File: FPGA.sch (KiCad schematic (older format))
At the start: 10 parts, among them U13 ADS1015, U14 SiT8008B, U8 GW1N-9LQ100

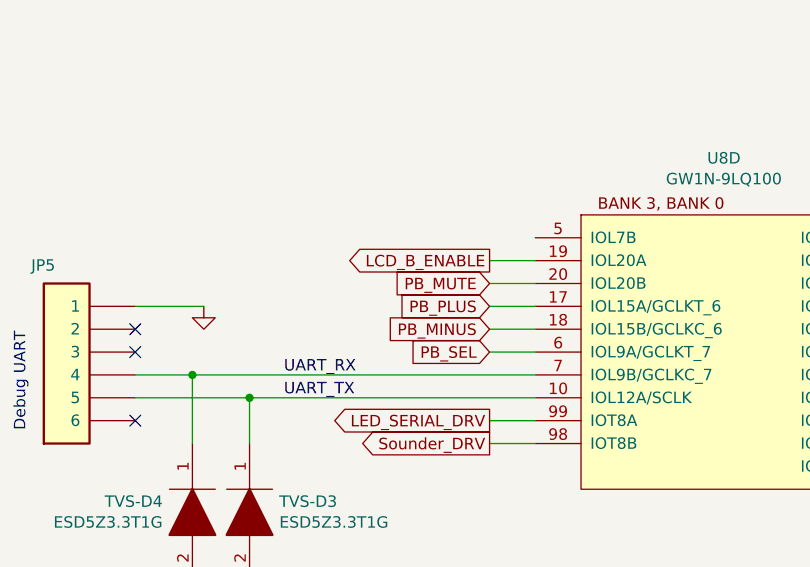
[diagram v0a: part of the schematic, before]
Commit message: Update FPGA.sch
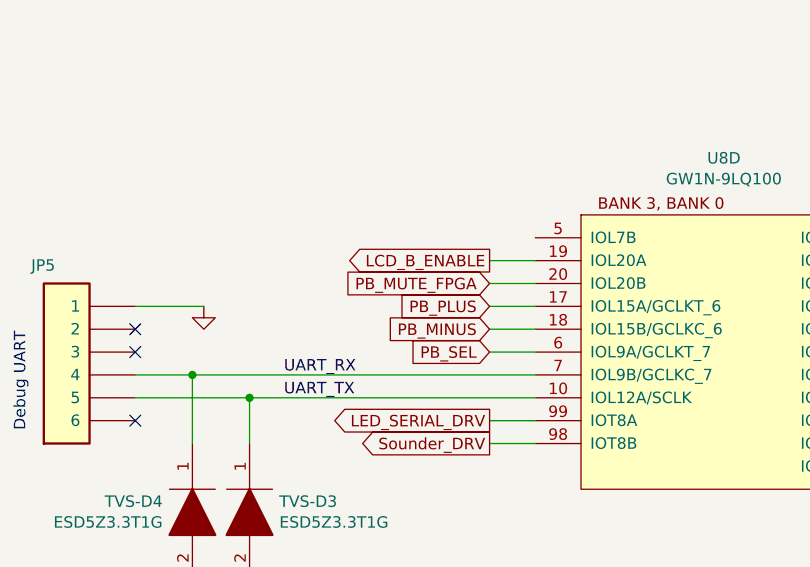
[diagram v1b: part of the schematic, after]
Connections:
- net labels added: PB_MUTE_FPGA
- net labels removed: PB_MUTE
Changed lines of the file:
@@
 Text GLabel 5550 7350 0    50   Output ~ 0
 Motor_off
-Text GLabel 7450 5050 0    50   Input ~ 0
-PB_MUTE
 Text GLabel 7450 5150 0    50   Input ~ 0
 PB_PLUS
@@
 Wire Wire Line
 	6300 6350 6400 6350
+Text GLabel 7450 5050 0    50   Input ~ 0
+PB_MUTE_FPGA
 $EndSCHEMATC

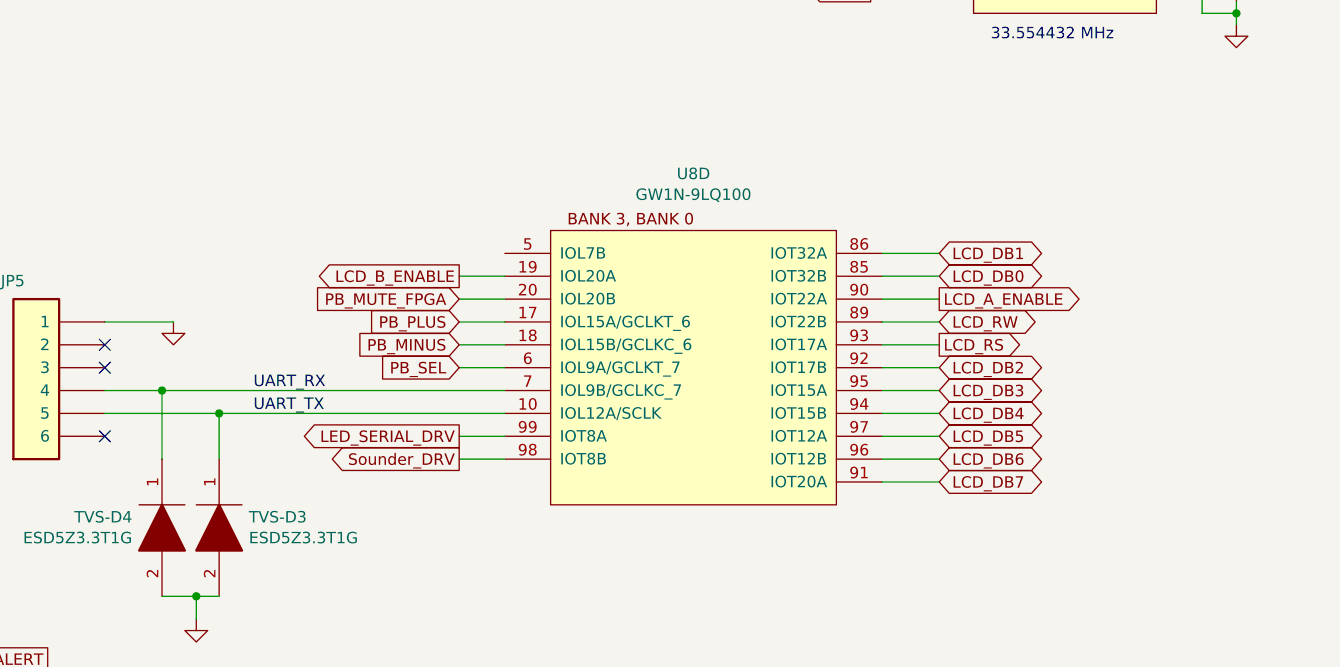
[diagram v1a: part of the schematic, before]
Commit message: Update FPGA.sch
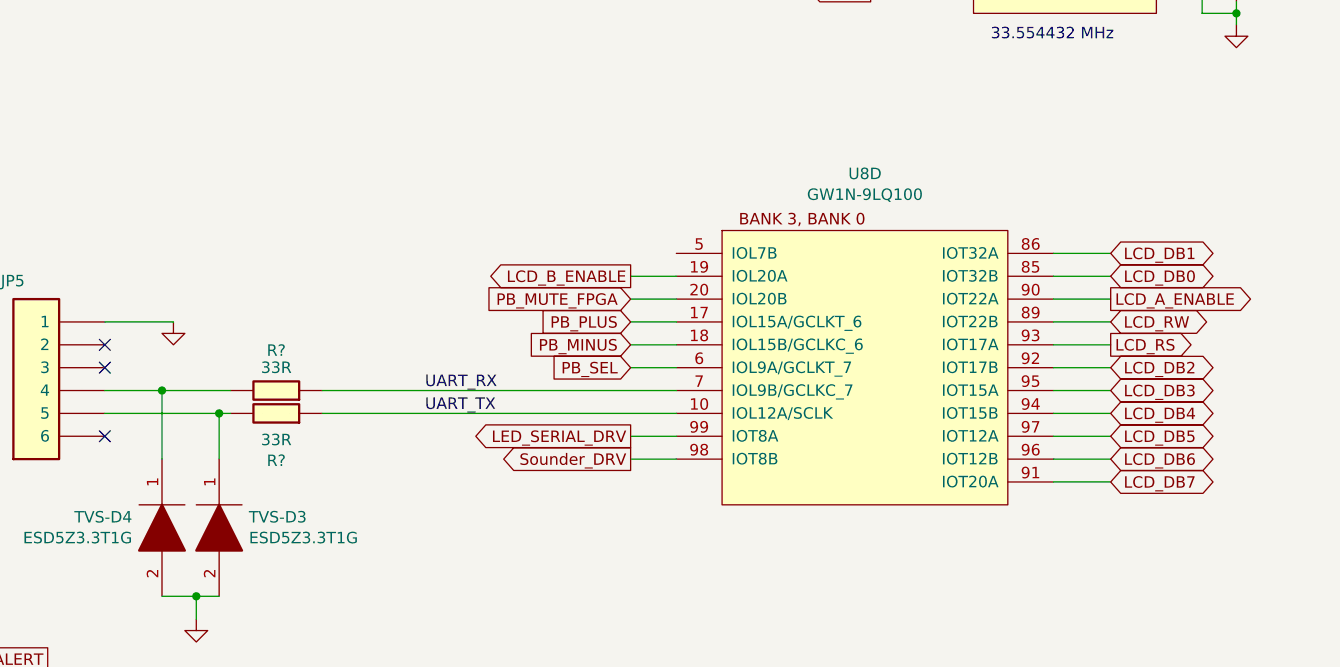
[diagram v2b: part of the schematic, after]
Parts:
- added R? (x2): 33R_Chip_Resistor,_1%,_0.1W, symbol OpenVent:33R_Chip_Resistor,_1%,_0.1W
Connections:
- wire segments 104 -> 106
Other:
- moved on the sheet: U8D
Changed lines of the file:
@@
 Text GLabel 5650 6625 0    50   Output ~ 0
 nPRESSURE-PATIENT-ALERT
-Text GLabel 7450 5750 0    50   Output ~ 0
+Text GLabel 8200 5750 0    50   Output ~ 0
 Sounder_DRV
 $Comp
@@
 Text GLabel 5550 7350 0    50   Output ~ 0
 Motor_off
-Text GLabel 7450 5150 0    50   Input ~ 0
+Text GLabel 8200 5150 0    50   Input ~ 0
 PB_PLUS
-Text GLabel 7450 5250 0    50   Input ~ 0
+Text GLabel 8200 5250 0    50   Input ~ 0
 PB_MINUS
-Text GLabel 7450 5350 0    50   Input ~ 0
+Text GLabel 8200 5350 0    50   Input ~ 0
 PB_SEL
 Text GLabel 9700 1200 2    50   Output ~ 0
@@
 Text GLabel 4450 4400 2    50   Input ~ 0
 Vcap_F
-Text GLabel 9550 5250 2    50   Output ~ 0
+Text GLabel 10300 5250 2    50   Output ~ 0
 LCD_RS
-Text GLabel 9550 5150 2    50   BiDi ~ 0
+Text GLabel 10300 5150 2    50   BiDi ~ 0
 LCD_RW
-Text GLabel 9550 5050 2    50   Output ~ 0
+Text GLabel 10300 5050 2    50   Output ~ 0
 LCD_A_ENABLE
-Text GLabel 9550 4950 2    50   BiDi ~ 0
+Text GLabel 10300 4950 2    50   BiDi ~ 0
 LCD_DB0
-Text GLabel 9550 4850 2    50   BiDi ~ 0
+Text GLabel 10300 4850 2    50   BiDi ~ 0
 LCD_DB1
-Text GLabel 9550 5450 2    50   BiDi ~ 0
+Text GLabel 10300 5450 2    50   BiDi ~ 0
 LCD_DB3
-Text GLabel 9550 5350 2    50   BiDi ~ 0
+Text GLabel 10300 5350 2    50   BiDi ~ 0
 LCD_DB2
-Text GLabel 9550 5650 2    50   BiDi ~ 0
+Text GLabel 10300 5650 2    50   BiDi ~ 0
 LCD_DB5
-Text GLabel 9550 5550 2    50   BiDi ~ 0
+Text GLabel 10300 5550 2    50   BiDi ~ 0
 LCD_DB4
-Text GLabel 9550 5850 2    50   BiDi ~ 0
+Text GLabel 10300 5850 2    50   BiDi ~ 0
 LCD_DB7
-Text GLabel 9550 5750 2    50   BiDi ~ 0
+Text GLabel 10300 5750 2    50   BiDi ~ 0
 LCD_DB6
 Wire Notes Line
@@
 $EndComp
 Wire Wire Line
-	9550 4850 9300 4850
-Wire Wire Line
-	9300 4950 9550 4950
-Wire Wire Line
-	9550 5050 9300 5050
-Wire Wire Line
-	9300 5150 9550 5150
-Wire Wire Line
-	9550 5250 9300 5250
-Wire Wire Line
-	9300 5350 9550 5350
-Wire Wire Line
-	9550 5450 9300 5450
-Wire Wire Line
-	9300 5550 9550 5550
-Wire Wire Line
-	9550 5650 9300 5650
-Wire Wire Line
-	9300 5750 9550 5750
-Wire Wire Line
-	9550 5850 9300 5850
-Wire Wire Line
-	7650 5750 7450 5750
-Wire Wire Line
-	7450 5650 7650 5650
+	10300 4850 10050 4850
+Wire Wire Line
+	10050 4950 10300 4950
+Wire Wire Line
+	10300 5050 10050 5050
+Wire Wire Line
+	10050 5150 10300 5150
+Wire Wire Line
+	10300 5250 10050 5250
+Wire Wire Line
+	10050 5350 10300 5350
+Wire Wire Line
+	10300 5450 10050 5450
+Wire Wire Line
+	10050 5550 10300 5550
+Wire Wire Line
+	10300 5650 10050 5650
+Wire Wire Line
+	10050 5750 10300 5750
+Wire Wire Line
+	10300 5850 10050 5850
+Wire Wire Line
+	8400 5750 8200 5750
+Wire Wire Line
+	8200 5650 8400 5650
 $Comp
 L OpenVent:100nF_0603_Ceramic_Capacitor,_10%,_X7R,_25V C23
@@
 Wire Wire Line
 	7000 2700 6650 2700
-Text GLabel 7450 4950 0    50   Output ~ 0
+Text GLabel 8200 4950 0    50   Output ~ 0
 LCD_B_ENABLE
 Wire Wire Line
-	7650 4950 7450 4950
+	8400 4950 8200 4950
 Wire Notes Line
 	500  2750 5250 2750
@@
 L OpenVent:GW1N-9LQ100 U8
 U 4 1 60544613
-P 8500 4750
-F 0 "U8" H 8475 4998 50  0000 C CNN
-F 1 "GW1N-9LQ100" H 8475 4907 50  0000 C CNN
-F 2 "" H 11800 3850 50  0001 C CNN
-F 3 "" H 11800 3850 50  0001 C CNN
-	4    8500 4750
+P 9250 4750
+F 0 "U8" H 9225 4998 50  0000 C CNN
+F 1 "GW1N-9LQ100" H 9225 4907 50  0000 C CNN
+F 2 "" H 12550 3850 50  0001 C CNN
+F 3 "" H 12550 3850 50  0001 C CNN
+	4    9250 4750
 	1    0    0    -1
 $EndComp
@@
 VBATT-SCALED
 Wire Wire Line
-	7450 5050 7650 5050
-Wire Wire Line
-	7450 5150 7650 5150
-Wire Wire Line
-	7450 5250 7650 5250
-Wire Wire Line
-	7450 5350 7650 5350
+	8200 5050 8400 5050
+Wire Wire Line
+	8200 5150 8400 5150
+Wire Wire Line
+	8200 5250 8400 5250
+Wire Wire Line
+	8200 5350 8400 5350
 Text Notes 5500 650  0    50   ~ 0
 I/Os ON BANKS 0, 2 AND 3 CAN BE FREELY INTERCHANGED AT LAYOUT EXCEPT CLCK WHICH MUST BE ON A GCLKT_x I/O PIN
@@
 	1    0    0    -1
 $EndComp
-Text Label 6550 5550 0    50   ~ 0
+Text Label 7300 5550 0    50   ~ 0
 UART_TX
-Text Label 6550 5450 0    50   ~ 0
+Text Label 7300 5450 0    50   ~ 0
 UART_RX
 $Comp
@@
 Text Notes 5425 5700 1    50   ~ 0
 Debug UART
-Text GLabel 7450 5650 0    50   Output ~ 0
+Text GLabel 8200 5650 0    50   Output ~ 0
 LED_SERIAL_DRV
 Wire Wire Line
@@
 Wire Wire Line
 	6400 5750 6400 5550
-Connection ~ 6400 5550
-Wire Wire Line
-	6400 5550 7650 5550
 Wire Wire Line
 	6150 5750 6150 5450
-Connection ~ 6150 5450
-Wire Wire Line
-	6150 5450 7650 5450
 Wire Wire Line
 	6150 6350 6300 6350
@@
 Wire Wire Line
 	6300 6350 6400 6350
-Text GLabel 7450 5050 0    50   Input ~ 0
+Text GLabel 8200 5050 0    50   Input ~ 0
 PB_MUTE_FPGA
+$Comp
+L OpenVent:33R_Chip_Resistor,_1%,_0.1W R?
+U 1 1 60586513
+P 6750 5650
+F 0 "R?" H 6850 5757 50  0000 C CNN
+F 1 "33R_Chip_Resistor,_1%,_0.1W" H 6400 6000 50  0001 C CNN
+F 2 "" H 6950 5650 50  0001 C CNN
+F 3 "" H 6750 5650 50  0001 C CNN
+F 4 "33R" H 6850 5666 50  0000 C CNN "Val"
+F 5 "1%" H 7300 5650 50  0001 C CNN "Tolerance"
+F 6 "0.1W" H 6750 5650 50  0001 C CNN "Watt"
+	1    6750 5650
+	-1   0    0    1
+$EndComp
+$Comp
+L OpenVent:33R_Chip_Resistor,_1%,_0.1W R?
+U 1 1 6058651C
+P 6750 5550
+F 0 "R?" H 6850 5275 50  0000 C CNN
+F 1 "33R_Chip_Resistor,_1%,_0.1W" H 6400 5900 50  0001 C CNN
+F 2 "" H 6950 5550 50  0001 C CNN
+F 3 "" H 6750 5550 50  0001 C CNN
+F 4 "33R" H 6850 5350 50  0000 C CNN "Val"
+F 5 "1%" H 7300 5550 50  0001 C CNN "Tolerance"
+F 6 "0.1W" H 6750 5550 50  0001 C CNN "Watt"
+	1    6750 5550
+	-1   0    0    1
+$EndComp
+Wire Wire Line
+	6850 5450 8400 5450
+Wire Wire Line
+	6850 5550 8400 5550
+Wire Wire Line
+	6450 5550 6400 5550
+Connection ~ 6400 5550
+Wire Wire Line
+	6450 5450 6150 5450
+Connection ~ 6150 5450
 $EndSCHEMATC
